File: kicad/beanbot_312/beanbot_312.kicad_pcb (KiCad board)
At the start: 2 copper layers, 100 x 100 mm, 45 parts, among them M1 >VALUE, M10 >VALUE, M11 >VALUE, M12 >VALUE, M13 >VALUE, M14 P&O2_MOSFET, M15 >VALUE, M16 P&O2_ULTRASONE_HC_SR04, M17 >VALUE, M18 >VALUE, M19 >VALUE, M2 >VALUE, M20 >VALUE, M21 P&O2_GEWICHTSENSOR2, M23 >VALUE, M24 >VALUE, M25 P&O2_KLEURSENSOR, M26 >VALUE, M27 >VALUE, M28 >VALUE, M29 P&O2_RELAIS-DP, M3 >VALUE, M30 P&O2_DC-MOTOR, M31 P&O2_RELAIS-DP, M32 P&O2_DC-MOTOR, M35 >VALUE, M36 >VALUE, M38 >VALUE, M39 >VALUE, M4 P&O2_MOSFET, M41 >VALUE, M42 >VALUE, M44 >VALUE, M45 >VALUE, M47 P&O2_MOSFET, M48 P&O2_MOSFET, M5 >VALUE, M50 >VALUE, M51 >VALUE, M6 >VALUE, M7 >VALUE, M8 P&O2_MOSFET, M9 >VALUE, U1 P&O2_ARDUINO_MEGA_SHIELD

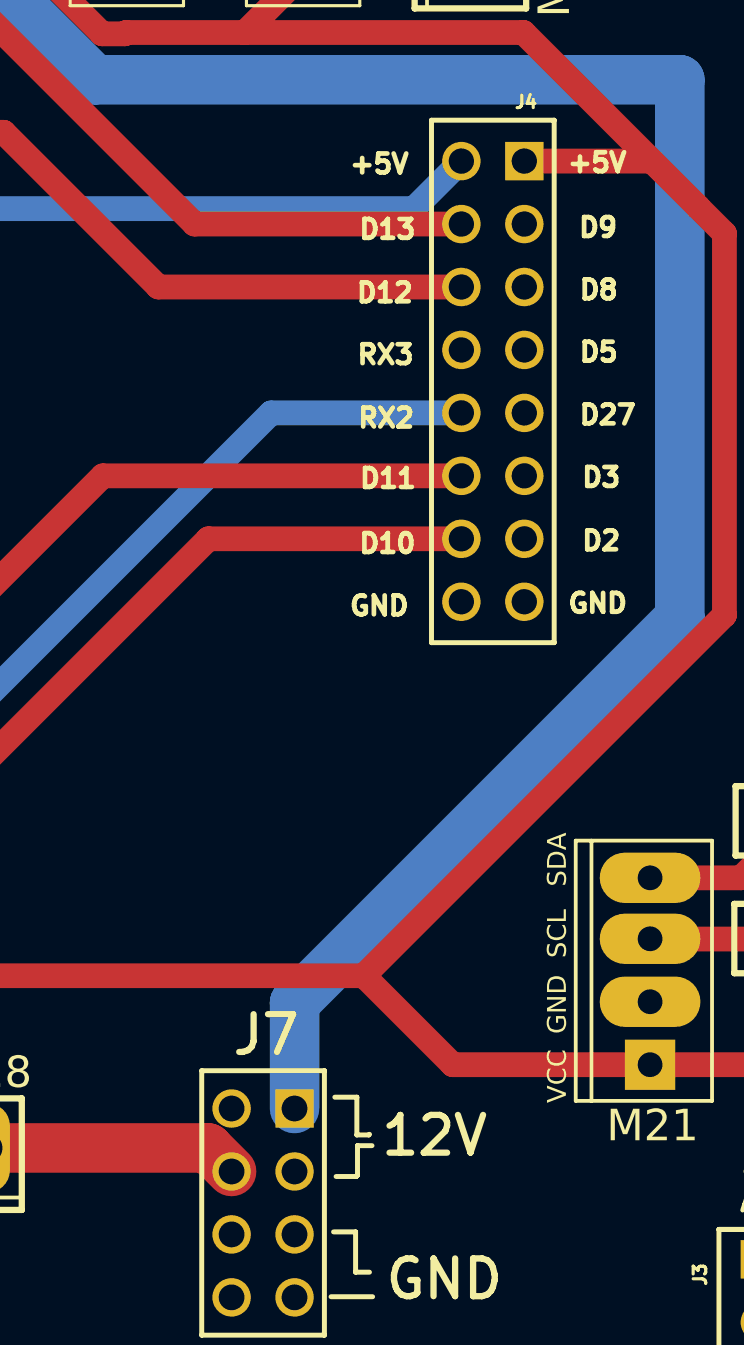
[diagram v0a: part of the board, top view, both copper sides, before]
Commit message: Cleared warnings
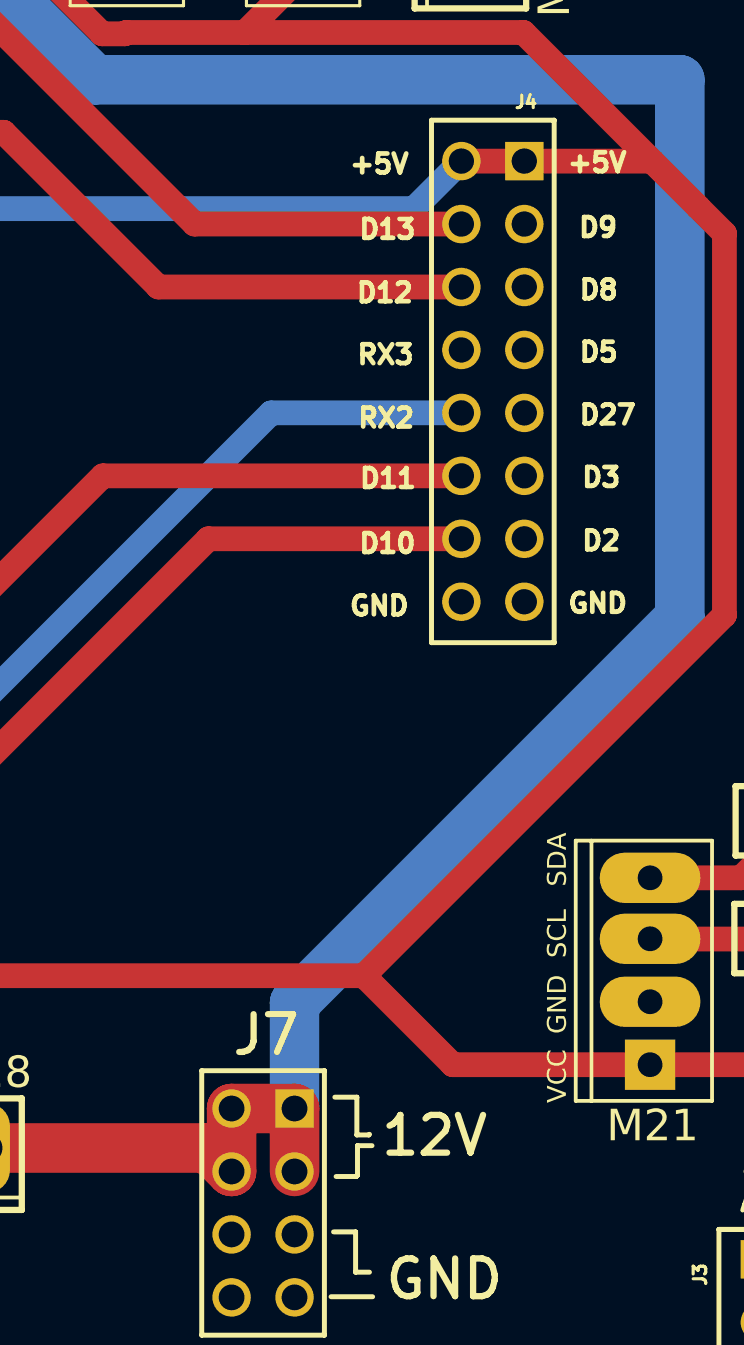
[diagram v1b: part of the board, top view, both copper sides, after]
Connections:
- U1 pad 2: unconnected-(U1-Pad2) -> /GND
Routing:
- net /12V: track 206.0 -> 213.6 mm
- net /5V: track 218.3 -> 220.9 mm
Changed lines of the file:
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@@
       (net 43 "unconnected-(U1-Pad2)") (pinfunction "GND") (pintype "bidirectional"))
     (pad "2" thru_hole circle (at 3.744999 -1.525001 270) (size 1.55 1.55) (drill 1.04) (layers *.Cu *.Mask)
-      (net 43 "unconnected-(U1-Pad2)") (pinfunction "GND") (pintype "bidirectional"))
+      (net 3 "/GND") (pinfunction "GND") (pintype "bidirectional"))
     (pad "2" thru_hole circle (at 33.234409 -46.076605 270) (size 1.55 1.55) (drill 1.02) (layers *.Cu *.Mask)
       (net 43 "unconnected-(U1-Pad2)") (pinfunction "GND") (pintype "bidirectional"))
@@
       (net 43 "unconnected-(U1-Pad2)") (pinfunction "GND") (pintype "bidirectional"))
     (pad "2" thru_hole circle (at 1.204999 -1.525001 270) (size 1.55 1.55) (drill 1.04) (layers *.Cu *.Mask)
-      (net 43 "unconnected-(U1-Pad2)") (pinfunction "GND") (pintype "bidirectional"))
+      (net 3 "/GND") (pinfunction "GND") (pintype "bidirectional"))
     (pad "2" thru_hole circle (at 10.476007 -29.591997 270) (size 1.55 1.55) (drill 1.02) (layers *.Cu *.Mask)
       (net 43 "unconnected-(U1-Pad2)") (pinfunction "GND") (pintype "bidirectional"))
     (pad "2" thru_hole circle (at 1.204999 -4.065001 270) (size 1.55 1.55) (drill 1.04) (layers *.Cu *.Mask)
-      (net 43 "unconnected-(U1-Pad2)") (pinfunction "GND") (pintype "bidirectional"))
+      (net 3 "/GND") (pinfunction "GND") (pintype "bidirectional"))
     (pad "2" thru_hole circle (at 13.016007 -29.591997 270) (size 1.55 1.55) (drill 1.02) (layers *.Cu *.Mask)
       (net 43 "unconnected-(U1-Pad2)") (pinfunction "GND") (pintype "bidirectional"))
@@
       (net 43 "unconnected-(U1-Pad2)") (pinfunction "GND") (pintype "bidirectional"))
     (pad "2" thru_hole circle (at 3.744999 -4.065001 270) (size 1.55 1.55) (drill 1.04) (layers *.Cu *.Mask)
-      (net 43 "unconnected-(U1-Pad2)") (pinfunction "GND") (pintype "bidirectional"))
+      (net 3 "/GND") (pinfunction "GND") (pintype "bidirectional"))
     (pad "3" thru_hole circle (at 22.519981 -0.521544) (size 1.55 1.55) (drill 1.02) (layers *.Cu *.Mask)
       (net 44 "unconnected-(U1-Pad3)") (pinfunction "A0") (pintype "bidirectional"))
@@
   (segment (start 126.724036 80.56) (end 124.888 82.396036) (width 1) (layer "F.Cu") (net 1))
   (segment (start 144.892655 87.992655) (end 133.647345 87.992655) (width 1) (layer "F.Cu") (net 1))
+  (segment (start 142.38561 93.18081) (end 144.92561 93.18081) (width 1) (layer "F.Cu") (net 1))
   (segment (start 142.04 129.64) (end 150 129.64) (width 1) (layer "F.Cu") (net 1))
   (segment (start 150 129.64) (end 171.64 129.64) (width 1) (layer "F.Cu") (net 1))
@@
   (segment (start 140.02542 57.4) (end 134.88192 62.5435) (width 2) (layer "F.Cu") (net 20))
   (segment (start 124.8032 70.1) (end 127.399711 67.503489) (width 2) (layer "F.Cu") (net 20))
+  (segment (start 133.114602 133.947806) (end 133.114602 131.407806) (width 2) (layer "F.Cu") (net 20))
   (segment (start 127.399711 67.503489) (end 129.921931 67.503489) (width 2) (layer "F.Cu") (net 20))
   (segment (start 164.2251 57.4) (end 169.1435 57.4) (width 2) (layer "F.Cu") (net 20))
   (segment (start 174.4435 52.1) (end 177.040011 54.696511) (width 2) (layer "F.Cu") (net 20))
+  (segment (start 135.654602 131.407806) (end 135.654602 133.947806) (width 2) (layer "F.Cu") (net 20))
   (segment (start 186.7 66.90158) (end 181.97714 62.17872) (width 2) (layer "F.Cu") (net 20))
   (segment (start 123.27 133) (end 132.166796 133) (width 2) (layer "F.Cu") (net 20))
@@
   (segment (start 133.114602 133.947806) (end 132.166796 133) (width 2) (layer "F.Cu") (net 20))
   (segment (start 186.7 91.53968) (end 186.7 66.90158) (width 2) (layer "F.Cu") (net 20))
+  (segment (start 133.114602 131.407806) (end 135.654602 131.407806) (width 2) (layer "F.Cu") (net 20))
   (segment (start 177.040011 54.696511) (end 177.040011 57.218731) (width 2) (layer "F.Cu") (net 20))
   (segment (start 164.2251 57.4) (end 140.02542 57.4) (width 2) (layer "F.Cu") (net 20))
